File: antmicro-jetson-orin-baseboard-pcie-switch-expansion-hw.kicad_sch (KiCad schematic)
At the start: 10 parts

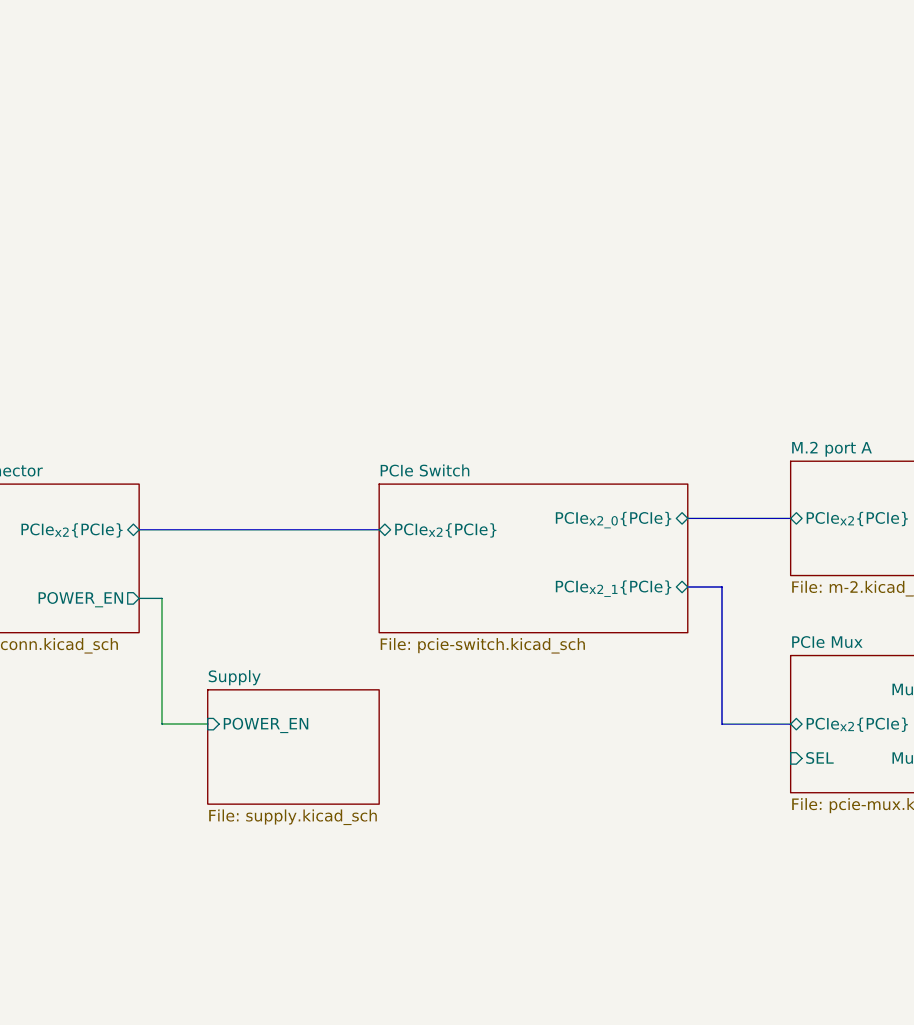
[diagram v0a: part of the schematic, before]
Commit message: [#100765] Work on schematic
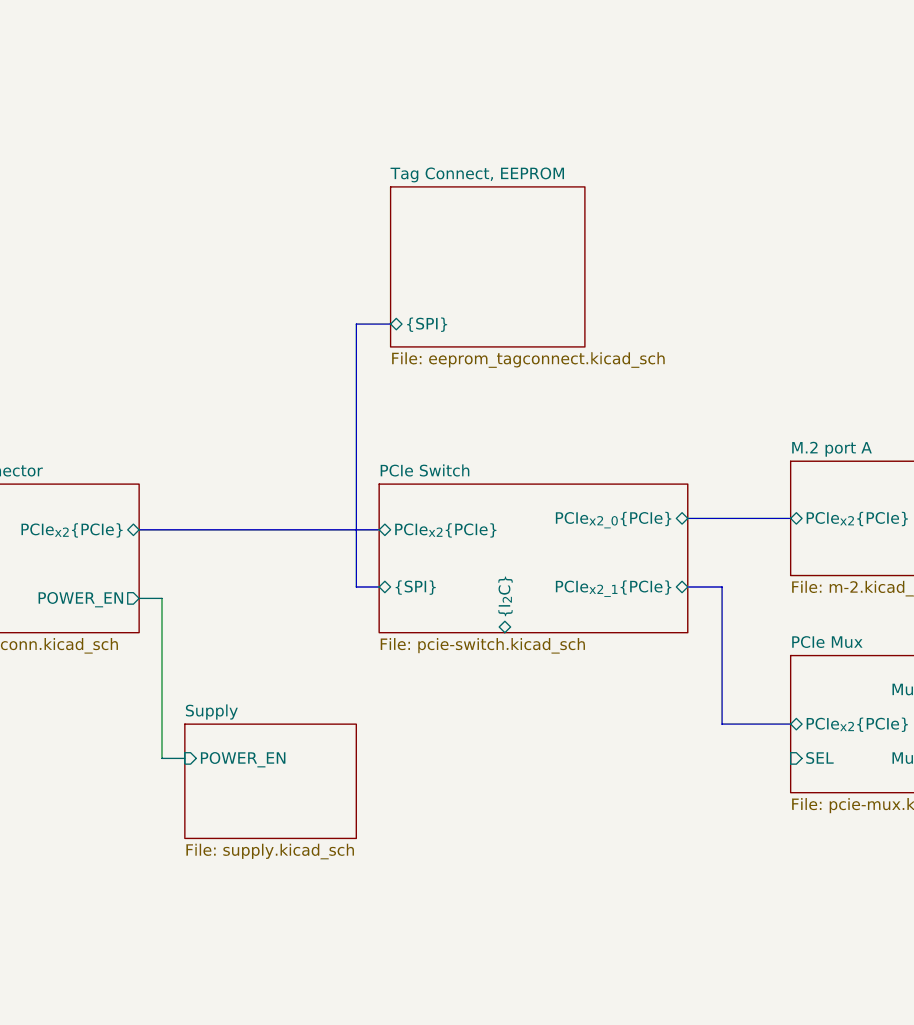
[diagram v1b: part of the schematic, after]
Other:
- added sheet Tag Connect, EEPROM (eeprom_tagconnect.kicad_sch)
- sheet PCIe Switch ports: added {I_{2}C}, {SPI}; removed none
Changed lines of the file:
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@@
 	(wire
 		(pts
-			(xy 232.41 113.03) (xy 237.49 113.03)
+			(xy 232.41 116.84) (xy 234.95 116.84)
 		)
 		(stroke
@@
 	(bus
 		(pts
+			(xy 254 97.79) (xy 256.54 97.79)
+		)
+		(stroke
+			(width 0)
+			(type default)
+		)
+	)
+	(bus
+		(pts
 			(xy 290.83 90.17) (xy 302.26 90.17)
 		)
@@
 		)
 	)
+	(bus
+		(pts
+			(xy 254 68.58) (xy 254 97.79)
+		)
+		(stroke
+			(width 0)
+			(type default)
+		)
+	)
 	(wire
 		(pts
@@
 		)
 	)
+	(bus
+		(pts
+			(xy 257.81 68.58) (xy 254 68.58)
+		)
+		(stroke
+			(width 0)
+			(type default)
+		)
+	)
 	(wire
 		(pts
-			(xy 232.41 99.06) (xy 232.41 113.03)
+			(xy 232.41 116.84) (xy 232.41 99.06)
 		)
 		(stroke
@@
 			)
 		)
+		(pin "{I_{2}C}" bidirectional
+			(at 270.51 102.87 270)
+			(effects
+				(font
+					(size 1.27 1.27)
+				)
+				(justify left)
+			)
+		)
+		(pin "{SPI}" bidirectional
+			(at 256.54 97.79 180)
+			(effects
+				(font
+					(size 1.27 1.27)
+				)
+				(justify left)
+			)
+		)
 		(instances
 			(project "antmicro-jetson-orin-baseboard-pcie-switch-expansion-hw"
@@
 	)
 	(sheet
+		(at 257.81 53.34)
+		(size 21.59 17.78)
+		(exclude_from_sim no)
+		(in_bom yes)
+		(on_board yes)
+		(dnp no)
+		(fields_autoplaced yes)
+		(stroke
+			(width 0.1524)
+			(type solid)
+		)
+		(fill
+			(color 0 0 0 0)
+		)
+		(property "Sheetname" "Tag Connect, EEPROM"
+			(at 257.81 52.6284 0)
+			(show_name no)
+			(do_not_autoplace no)
+			(effects
+				(font
+					(size 1.27 1.27)
+				)
+				(justify left bottom)
+			)
+		)
+		(property "Sheetfile" "eeprom_tagconnect.kicad_sch"
+			(at 257.81 71.7046 0)
+			(show_name no)
+			(do_not_autoplace no)
+			(effects
+				(font
+					(size 1.27 1.27)
+				)
+				(justify left top)
+			)
+		)
+		(pin "{SPI}" bidirectional
+			(at 257.81 68.58 180)
+			(effects
+				(font
+					(size 1.27 1.27)
+				)
+				(justify left)
+			)
+		)
+		(instances
+			(project "antmicro-jetson-orin-baseboard-pcie-switch-expansion-hw"
+				(path "/9f8272ef-d62d-4578-9094-a2852fcd4bf4"
+					(page "9")
+				)
+			)
+		)
+	)
+	(sheet
 		(at 302.26 105.41)
 		(size 30.48 15.24)
@@
 	)
 	(sheet
-		(at 237.49 109.22)
+		(at 234.95 113.03)
 		(size 19.05 12.7)
 		(exclude_from_sim no)
@@
 		)
 		(property "Sheetname" "Supply"
-			(at 237.49 108.5084 0)
+			(at 234.95 112.3184 0)
 			(show_name no)
 			(do_not_autoplace no)
@@
 		)
 		(property "Sheetfile" "supply.kicad_sch"
-			(at 237.49 122.5046 0)
+			(at 234.95 126.3146 0)
 			(show_name no)
 			(do_not_autoplace no)
@@
 		)
 		(pin "POWER_EN" input
-			(at 237.49 113.03 180)
-			(effects
-				(font
+			(at 234.95 116.84 180)
+			(effects
+				(font

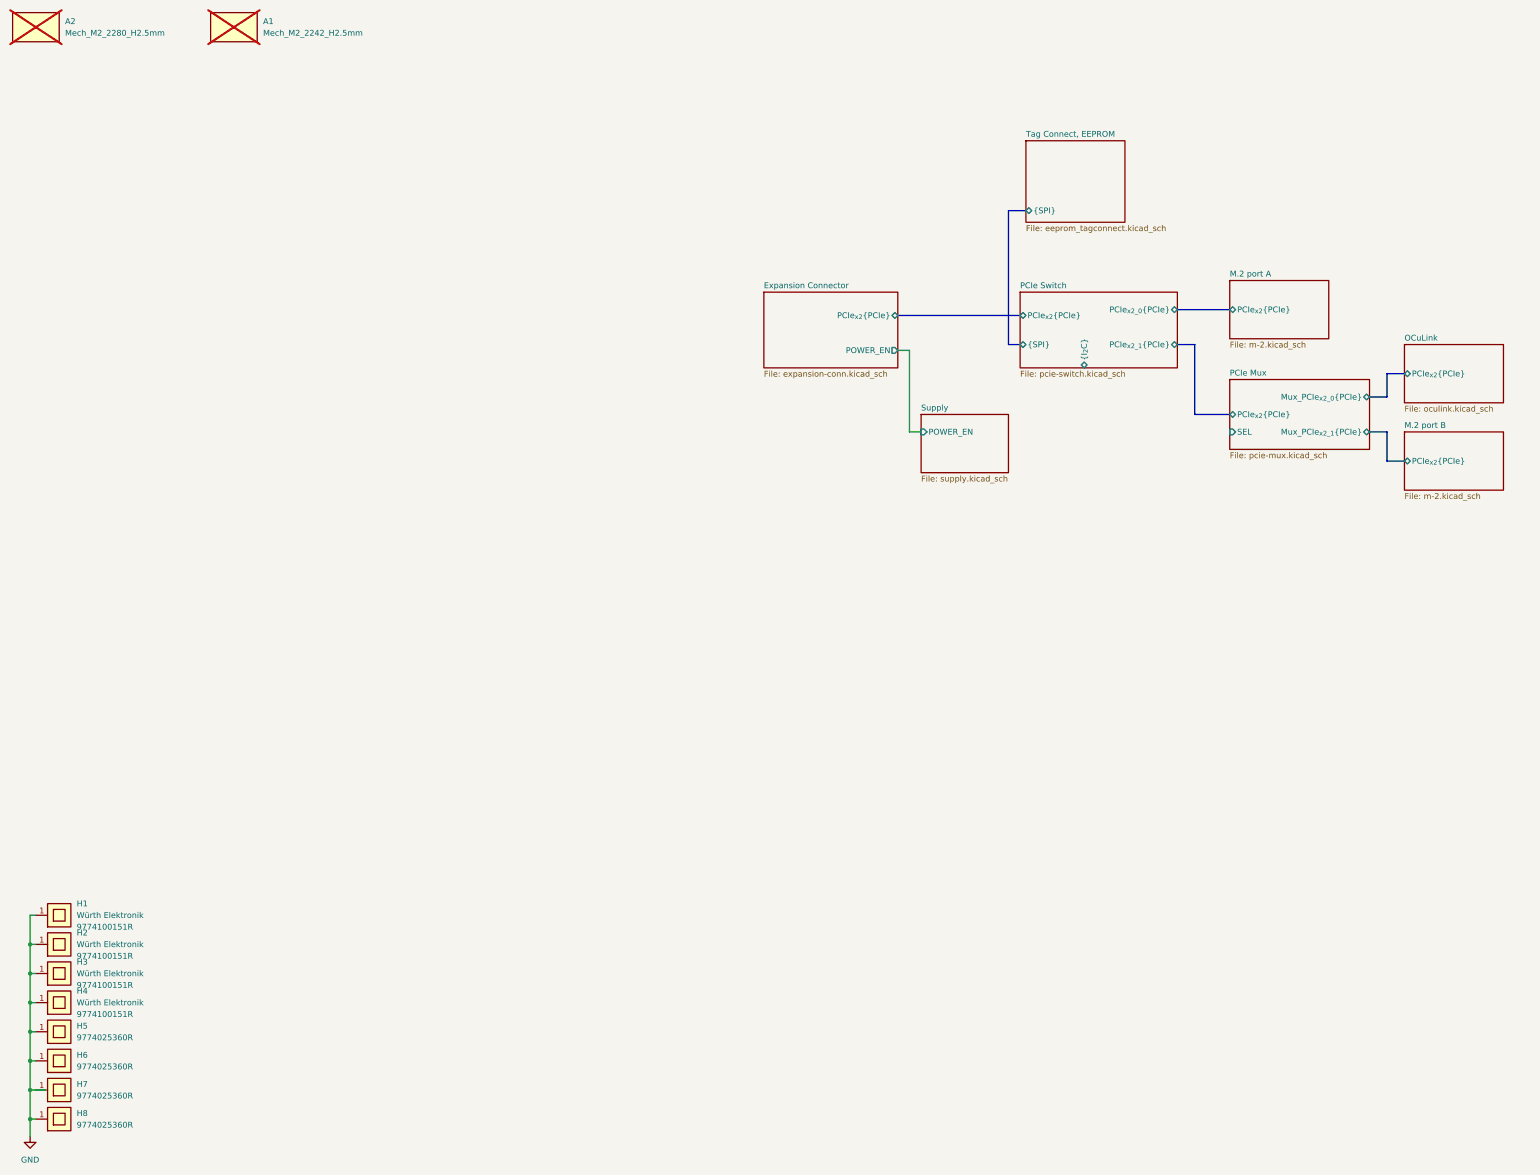
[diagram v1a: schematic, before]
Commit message: [#100765] Update schematic
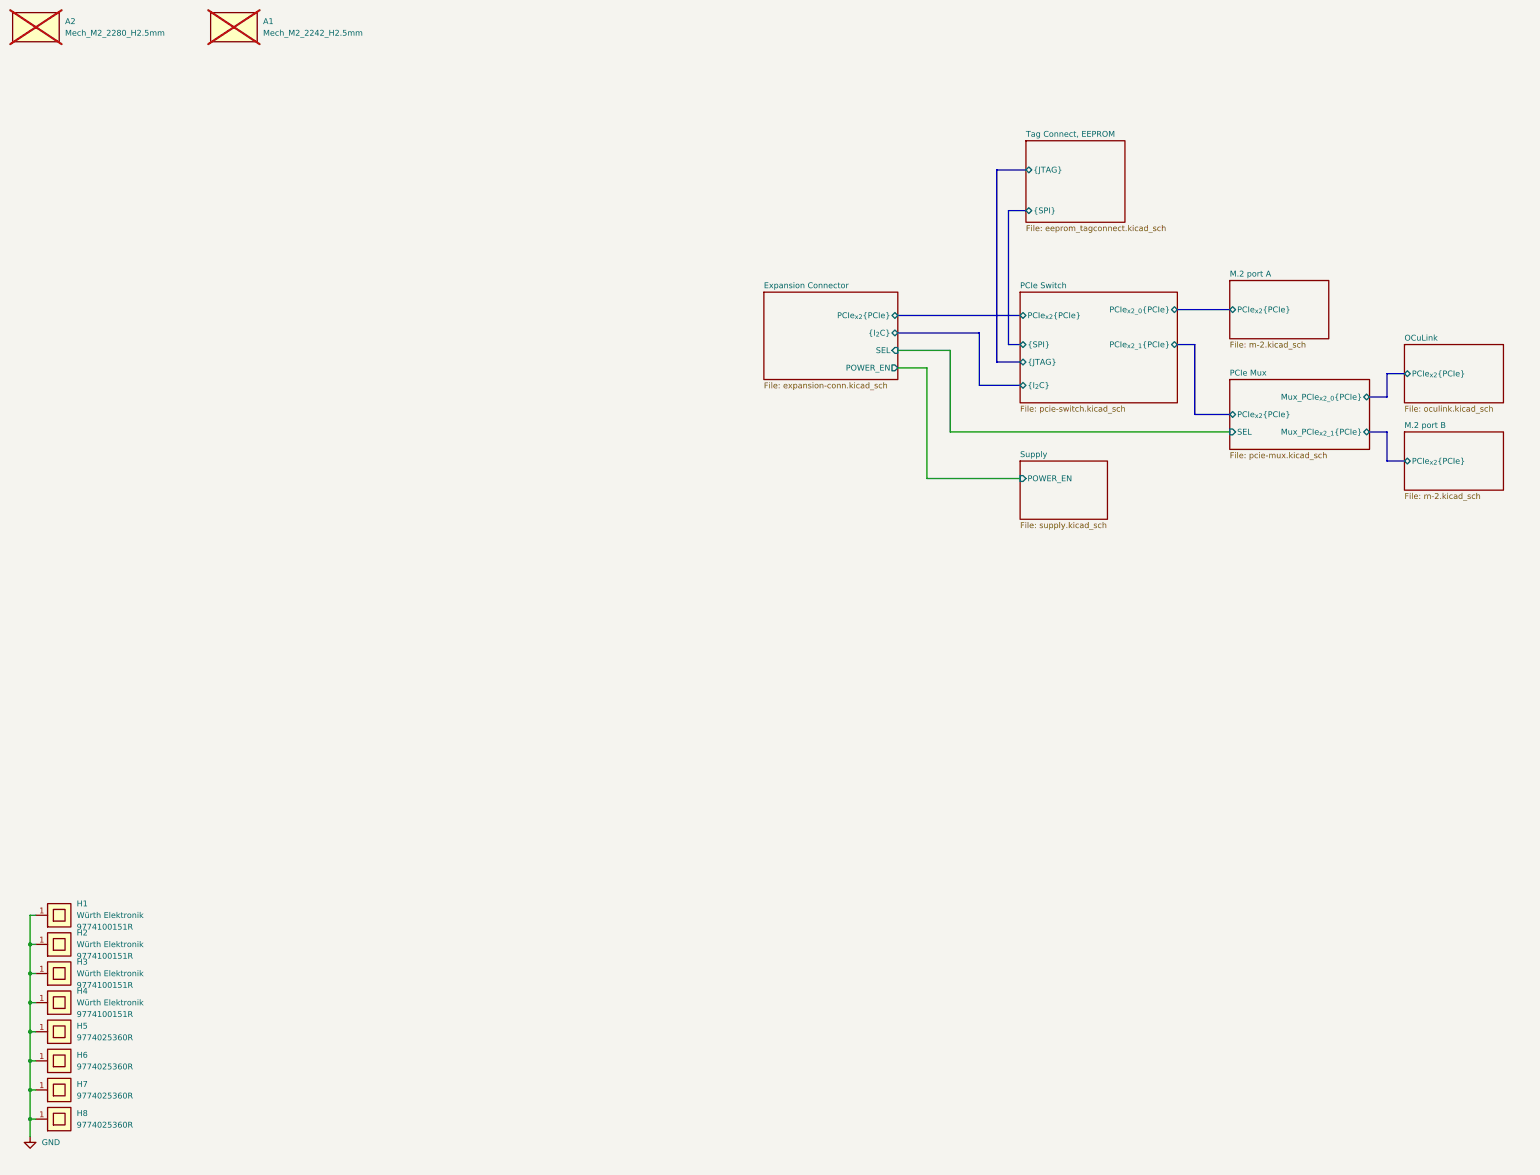
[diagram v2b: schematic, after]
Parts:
- A2: now left out of the parts list
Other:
- sheet Expansion Connector ports: added SEL, {I_{2}C}; removed none
- sheet PCIe Switch ports: added {JTAG}; removed none
- sheet Tag Connect, EEPROM ports: added {JTAG}; removed none
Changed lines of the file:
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@@
 	(wire
 		(pts
-			(xy 229.87 99.06) (xy 232.41 99.06)
+			(xy 229.87 102.87) (xy 236.22 102.87)
+		)
+		(stroke
+			(width 0)
+			(type default)
+		)
+	)
+	(bus
+		(pts
+			(xy 251.46 101.6) (xy 256.54 101.6)
 		)
 		(stroke
@@
 	(bus
 		(pts
+			(xy 247.65 95.25) (xy 247.65 106.68)
+		)
+		(stroke
+			(width 0)
+			(type default)
+		)
+	)
+	(bus
+		(pts
 			(xy 332.74 116.84) (xy 336.55 116.84)
 		)
@@
 		)
 	)
+	(bus
+		(pts
+			(xy 247.65 106.68) (xy 256.54 106.68)
+		)
+		(stroke
+			(width 0)
+			(type default)
+		)
+	)
 	(wire
 		(pts
-			(xy 232.41 116.84) (xy 234.95 116.84)
+			(xy 236.22 127) (xy 256.54 127)
 		)
 		(stroke
@@
 		)
 	)
+	(bus
+		(pts
+			(xy 251.46 59.69) (xy 251.46 101.6)
+		)
+		(stroke
+			(width 0)
+			(type default)
+		)
+	)
+	(bus
+		(pts
+			(xy 290.83 97.79) (xy 294.64 97.79)
+		)
+		(stroke
+			(width 0)
+			(type default)
+		)
+	)
 	(wire
 		(pts
-			(xy 44.1451 260.35) (xy 41.91 260.35)
+			(xy 241.3 99.06) (xy 241.3 116.84)
 		)
 		(stroke
@@
 	(bus
 		(pts
-			(xy 290.83 97.79) (xy 294.64 97.79)
+			(xy 229.87 95.25) (xy 247.65 95.25)
 		)
 		(stroke
@@
 	(bus
 		(pts
+			(xy 257.81 59.69) (xy 251.46 59.69)
+		)
+		(stroke
+			(width 0)
+			(type default)
+		)
+	)
+	(bus
+		(pts
 			(xy 294.64 113.03) (xy 302.26 113.03)
 		)
@@
 	(wire
 		(pts
+			(xy 229.87 99.06) (xy 241.3 99.06)
+		)
+		(stroke
+			(width 0)
+			(type default)
+		)
+	)
+	(wire
+		(pts
+			(xy 241.3 116.84) (xy 302.26 116.84)
+		)
+		(stroke
+			(width 0)
+			(type default)
+		)
+	)
+	(wire
+		(pts
 			(xy 40.64 254) (xy 41.91 254)
 		)
@@
 	(wire
 		(pts
-			(xy 232.41 116.84) (xy 232.41 99.06)
+			(xy 236.22 127) (xy 236.22 102.87)
 		)
 		(stroke
@@
 		(body_style 1)
 		(exclude_from_sim no)
-		(in_bom yes)
+		(in_bom no)
 		(on_board yes)
 		(in_pos_files yes)
@@
 		)
 		(property "Value" "GND"
-			(at 40.64 275.59 0)
-			(show_name no)
-			(do_not_autoplace no)
-			(effects
-				(font
-					(size 1.27 1.27)
-					(thickness 0.15)
-				)
+			(at 43.18 271.78 0)
+			(show_name no)
+			(do_not_autoplace no)
+			(effects
+				(font
+					(size 1.27 1.27)
+					(thickness 0.15)
+				)
+				(justify left)
 			)
 		)
@@
 	(sheet
 		(at 256.54 86.36)
-		(size 34.29 16.51)
+		(size 34.29 24.13)
 		(exclude_from_sim no)
 		(in_bom yes)
@@
 		)
 		(property "Sheetfile" "pcie-switch.kicad_sch"
-			(at 256.54 103.4546 0)
+			(at 256.54 111.0746 0)
 			(show_name no)
 			(do_not_autoplace no)
@@
 		)
 		(pin "{I_{2}C}" bidirectional
-			(at 270.51 102.87 270)
+			(at 256.54 106.68 180)
 			(effects
 				(font
@@
 		(pin "{SPI}" bidirectional
 			(at 256.54 97.79 180)
+			(effects
+				(font
+					(size 1.27 1.27)
+				)
+				(justify left)
+			)
+		)
+		(pin "{JTAG}" bidirectional
+			(at 256.54 101.6 180)
 			(effects
 				(font
@@
 			)
 		)
+		(pin "{JTAG}" bidirectional
+			(at 257.81 59.69 180)
+			(effects
+				(font
+					(size 1.27 1.27)
+				)
+				(justify left)
+			)
+		)
 		(instances
 			(project "antmicro-jetson-orin-baseboard-pcie-switch-expansion-hw"
@@
 	)
 	(sheet
-		(at 234.95 113.03)
+		(at 256.54 123.19)
 		(size 19.05 12.7)
 		(exclude_from_sim no)
@@
 		)
 		(property "Sheetname" "Supply"
-			(at 234.95 112.3184 0)
+			(at 256.54 122.4784 0)
 			(show_name no)
 			(do_not_autoplace no)
@@
 		)
 		(property "Sheetfile" "supply.kicad_sch"
-			(at 234.95 126.3146 0)
+			(at 256.54 136.4746 0)
 			(show_name no)
 			(do_not_autoplace no)
@@
 		)
 		(pin "POWER_EN" input
-			(at 234.95 116.84 180)
+			(at 256.54 127 180)
 			(effects
 				(font
@@
 	(sheet
 		(at 200.66 86.36)
-		(size 29.21 16.51)
+		(size 29.21 19.05)
 		(exclude_from_sim no)
 		(in_bom yes)
@@
 		)
 		(property "Sheetfile" "expansion-conn.kicad_sch"
-			(at 200.66 103.4546 0)
+			(at 200.66 105.9946 0)
 			(show_name no)
 			(do_not_autoplace no)
@@
 		)
 		(pin "POWER_EN" output
-			(at 229.87 99.06 0)
+			(at 229.87 102.87 0)
 			(effects
 				(font
@@
 			(effects
 				(font
+					(size 1.27 1.27)
+				)
+				(justify right)
+			)
+		)
+		(pin "{I_{2}C}" bidirectional
+			(at 229.87 95.25 0)
+			(effects
+				(font
+					(size 1.27 1.27)
+				)
+				(justify right)
+			)
+		)
+		(pin "SEL" input
+			(at 229.87 99.06 0)
+			(effects
+				(font
